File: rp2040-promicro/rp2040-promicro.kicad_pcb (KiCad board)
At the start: 2 copper layers, 17.8 x 35.6 mm, 32 parts, among them J1 USB2.0_C_v3, J2 ProMicro-LeftPin, J3 ProMicro-RightPin, SW1 SW_Push, U1 RP2040, U2 W25Q128JVS, U3 AZ1117-3.3, Y1 Crystal_GND24

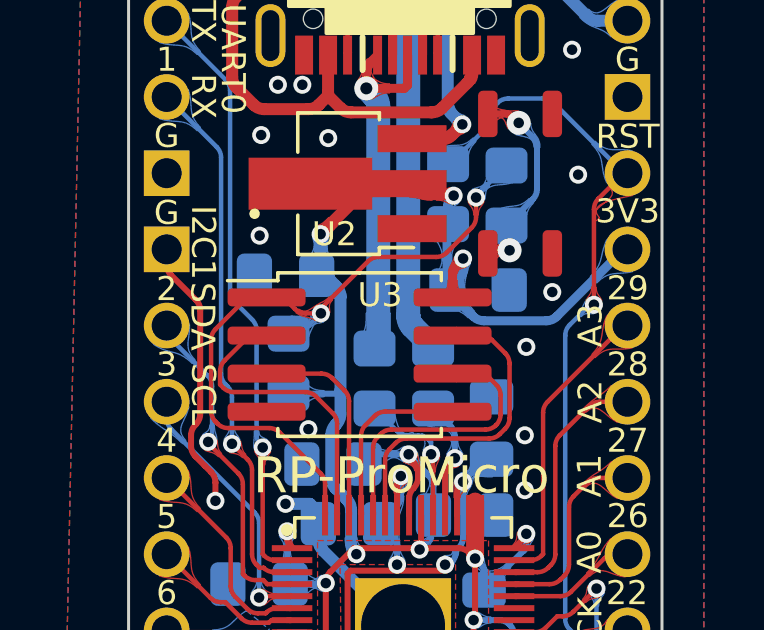
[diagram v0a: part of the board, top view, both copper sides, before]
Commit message: rp-promicro v2.0.0
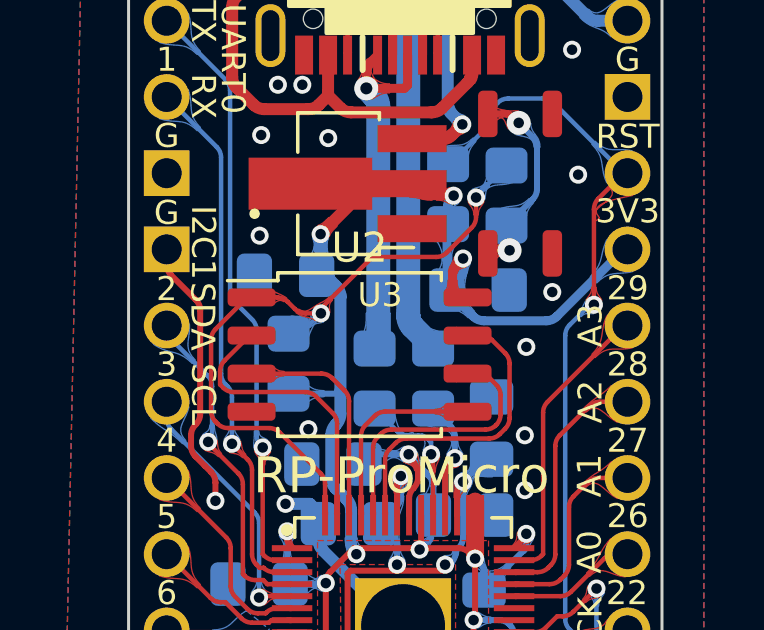
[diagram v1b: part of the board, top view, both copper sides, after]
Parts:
- U2: footprint rp2040-dev-board:W25Q16-128JV-SOIC -> Package_SO:SOIC-8_5.23x5.23mm_P1.27mm
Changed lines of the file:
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@@
     (descr "RP 2040")
     (tags "Integrated Circuit")
+    (property "MPN" "C2040")
     (property "Sheetfile" "rp2040-promicro.kicad_sch")
     (property "Sheetname" "")
@@
       (net 11 "9{slash}RX1") (pinfunction "9/A9") (pintype "bidirectional"))
   )
-  (footprint "rp2040-dev-board:W25Q16-128JV-SOIC" (layer "F.Cu")
+  (footprint "Package_SO:SOIC-8_5.23x5.23mm_P1.27mm" (layer "F.Cu")
     (at 57.7 62.397)
     (descr "SOIC, 8 Pin (http://www.winbond.com/resource-files/w25q32jv%20revg%2003272018%20plus.pdf#page=68), generated with kicad-footprint-generator ipc_gullwing_generator.py")
@@
     (property "Sheetname" "")
     (attr smd)
-    (fp_text reference "U2" (at -0.842 -4.015) (layer "F.SilkS")
-      (effects (font (size 0.8 0.8) (thickness 0.12)))
+    (fp_text reference "U2" (at 0 -3.56) (layer "F.SilkS")
+      (effects (font (size 1 1) (thickness 0.15)))
     )
     (fp_text value "W25Q128JVS" (at 0 3.56) (layer "F.Fab")
@@
       (effects (font (size 1 1) (thickness 0.15)))
     )
+    (fp_line (start -2.725 -2.725) (end -2.725 -2.465) (layer "F.SilkS") (width 0.12))
+    (fp_line (start 2.725 -2.725) (end 2.725 -2.465) (layer "F.SilkS") (width 0.12))
+    (fp_line (start 0 2.725) (end -2.725 2.725) (layer "F.SilkS") (width 0.12))
+    (fp_line (start -2.725 2.725) (end -2.725 2.465) (layer "F.SilkS") (width 0.12))
+    (fp_line (start -2.725 -2.465) (end -4.4 -2.465) (layer "F.SilkS") (width 0.12))
+    (fp_line (start 0 -2.725) (end -2.725 -2.725) (layer "F.SilkS") (width 0.12))
+    (fp_line (start 0 -2.725) (end 2.725 -2.725) (layer "F.SilkS") (width 0.12))
+    (fp_line (start 0 2.725) (end 2.725 2.725) (layer "F.SilkS") (width 0.12))
     (fp_line (start 2.725 2.725) (end 2.725 2.465) (layer "F.SilkS") (width 0.12))
-    (fp_line (start -2.725 -2.465) (end -4.4 -2.465) (layer "F.SilkS") (width 0.12))
-    (fp_line (start 0 -2.725) (end 2.725 -2.725) (layer "F.SilkS") (width 0.12))
-    (fp_line (start -2.725 2.725) (end -2.725 2.465) (layer "F.SilkS") (width 0.12))
-    (fp_line (start 2.725 -2.725) (end 2.725 -2.465) (layer "F.SilkS") (width 0.12))
-    (fp_line (start 0 -2.725) (end -2.725 -2.725) (layer "F.SilkS") (width 0.12))
-    (fp_line (start 0 2.725) (end -2.725 2.725) (layer "F.SilkS") (width 0.12))
-    (fp_line (start -2.725 -2.725) (end -2.725 -2.465) (layer "F.SilkS") (width 0.12))
-    (fp_line (start 0 2.725) (end 2.725 2.725) (layer "F.SilkS") (width 0.12))
+    (fp_line (start 4.65 2.86) (end 4.65 -2.86) (layer "F.CrtYd") (width 0.05))
+    (fp_line (start -4.65 2.86) (end 4.65 2.86) (layer "F.CrtYd") (width 0.05))
+    (fp_line (start 4.65 -2.86) (end -4.65 -2.86) (layer "F.CrtYd") (width 0.05))
     (fp_line (start -4.65 -2.86) (end -4.65 2.86) (layer "F.CrtYd") (width 0.05))
-    (fp_line (start 4.65 -2.86) (end -4.65 -2.86) (layer "F.CrtYd") (width 0.05))
-    (fp_line (start -4.65 2.86) (end 4.65 2.86) (layer "F.CrtYd") (width 0.05))
-    (fp_line (start 4.65 2.86) (end 4.65 -2.86) (layer "F.CrtYd") (width 0.05))
+    (fp_line (start -2.615 2.615) (end -2.615 -1.615) (layer "F.Fab") (width 0.1))
+    (fp_line (start 2.615 2.615) (end -2.615 2.615) (layer "F.Fab") (width 0.1))
     (fp_line (start -2.615 -1.615) (end -1.615 -2.615) (layer "F.Fab") (width 0.1))
+    (fp_line (start -1.615 -2.615) (end 2.615 -2.615) (layer "F.Fab") (width 0.1))
     (fp_line (start 2.615 -2.615) (end 2.615 2.615) (layer "F.Fab") (width 0.1))
-    (fp_line (start 2.615 2.615) (end -2.615 2.615) (layer "F.Fab") (width 0.1))
-    (fp_line (start -1.6 2.615) (end -1.6 -2.615) (layer "F.Fab") (width 0.1))
-    (fp_line (start -2.615 2.615) (end -2.615 -1.615) (layer "F.Fab") (width 0.1))
-    (fp_line (start -1.615 -2.615) (end 2.615 -2.615) (layer "F.Fab") (width 0.1))
-    (fp_line (start 1.6 2.615) (end 1.6 -2.615) (layer "F.Fab") (width 0.1))
-    (pad "1" smd roundrect (at -3.1 -1.905) (size 2.6 0.6) (layers "F.Cu" "F.Paste" "F.Mask") (roundrect_rratio 0.25)
+    (pad "1" smd roundrect locked (at -3.6 -1.905) (size 1.6 0.6) (layers "F.Cu" "F.Paste" "F.Mask") (roundrect_rratio 0.25)
       (net 1 "QSPI_SS") (pinfunction "~{CS}") (pintype "input"))
-    (pad "2" smd roundrect (at -3.1 -0.635) (size 2.6 0.6) (layers "F.Cu" "F.Paste" "F.Mask") (roundrect_rratio 0.25)
+    (pad "2" smd roundrect locked (at -3.6 -0.635) (size 1.6 0.6) (layers "F.Cu" "F.Paste" "F.Mask") (roundrect_rratio 0.25)
       (net 2 "QSPI_SD1") (pinfunction "DO(IO1)") (pintype "bidirectional"))
-    (pad "3" smd roundrect (at -3.1 0.635) (size 2.6 0.6) (layers "F.Cu" "F.Paste" "F.Mask") (roundrect_rratio 0.25)
+    (pad "3" smd roundrect locked (at -3.6 0.635) (size 1.6 0.6) (layers "F.Cu" "F.Paste" "F.Mask") (roundrect_rratio 0.25)
       (net 3 "QSPI_SD2") (pinfunction "IO2") (pintype "bidirectional"))
-    (pad "4" smd roundrect (at -3.1 1.905) (size 2.6 0.6) (layers "F.Cu" "F.Paste" "F.Mask") (roundrect_rratio 0.25)
-      (net 4 "GND") (pinfunction "GND") (pintype "power_in") (zone_connect 2))
-    (pad "5" smd roundrect (at 3.1 1.905) (size 2.6 0.6) (layers "F.Cu" "F.Paste" "F.Mask") (roundrect_rratio 0.25)
+    (pad "4" smd roundrect locked (at -3.6 1.905) (size 1.6 0.6) (layers "F.Cu" "F.Paste" "F.Mask") (roundrect_rratio 0.25)
+      (net 4 "GND") (pinfunction "GND") (pintype "power_in"))
+    (pad "5" smd roundrect locked (at 3.6 1.905) (size 1.6 0.6) (layers "F.Cu" "F.Paste" "F.Mask") (roundrect_rratio 0.25)
       (net 5 "QSPI_SD0") (pinfunction "DI(IO0)") (pintype "bidirectional"))
-    (pad "6" smd roundrect (at 3.1 0.635) (size 2.6 0.6) (layers "F.Cu" "F.Paste" "F.Mask") (roundrect_rratio 0.25)
+    (pad "6" smd roundrect locked (at 3.6 0.635) (size 1.6 0.6) (layers "F.Cu" "F.Paste" "F.Mask") (roundrect_rratio 0.25)
       (net 6 "QSPI_CLK") (pinfunction "CLK") (pintype "input"))
-    (pad "7" smd roundrect (at 3.1 -0.635) (size 2.6 0.6) (layers "F.Cu" "F.Paste" "F.Mask") (roundrect_rratio 0.25)
+    (pad "7" smd roundrect locked (at 3.6 -0.635) (size 1.6 0.6) (layers "F.Cu" "F.Paste" "F.Mask") (roundrect_rratio 0.25)
       (net 7 "QSPI_SD3") (pinfunction "IO3") (pintype "bidirectional"))
-    (pad "8" smd roundrect (at 3.1 -1.905) (size 2.6 0.6) (layers "F.Cu" "F.Paste" "F.Mask") (roundrect_rratio 0.25)
+    (pad "8" smd roundrect locked (at 3.6 -1.905) (size 1.6 0.6) (layers "F.Cu" "F.Paste" "F.Mask") (roundrect_rratio 0.25)
       (net 45 "+3V3") (pinfunction "VCC") (pintype "power_in"))
-    (model "${KICAD6_3DMODEL_DIR}/Package_SO.3dshapes/SOIC-8_5.275x5.275mm_P1.27mm.wrl"
+    (model "${KICAD6_3DMODEL_DIR}/Package_SO.3dshapes/SOIC-8_5.23x5.23mm_P1.27mm.wrl"
       (offset (xyz 0 0 0))
       (scale (xyz 1 1 1))

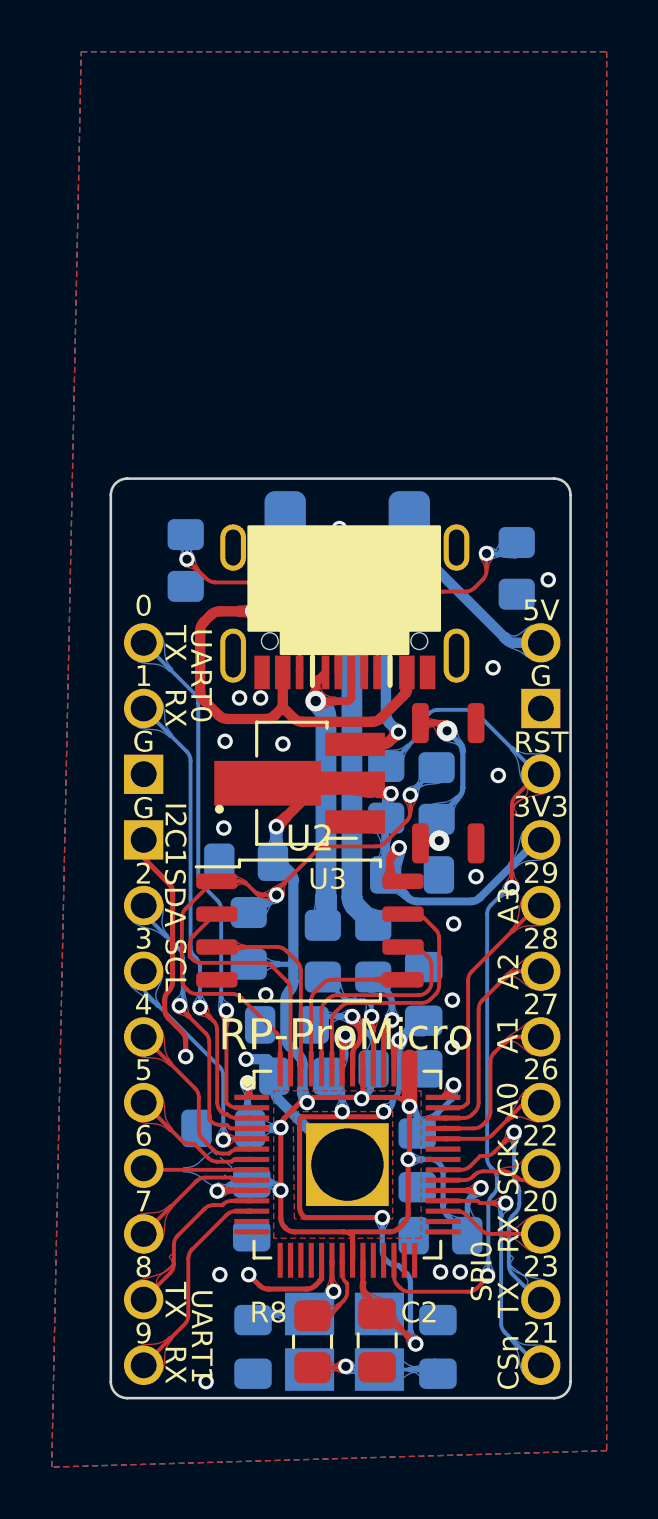
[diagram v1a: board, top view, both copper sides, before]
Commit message: rp-promicro v2.0.0
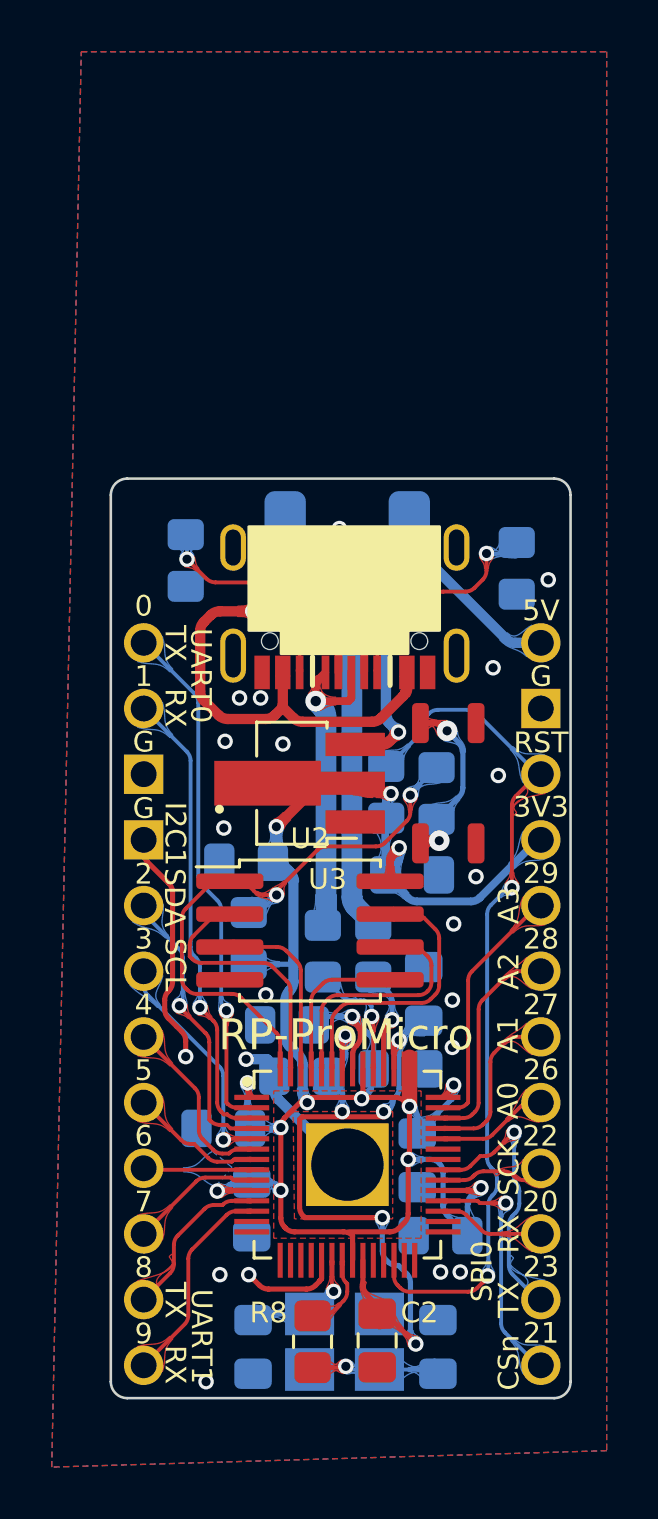
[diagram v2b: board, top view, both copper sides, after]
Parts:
- U2: footprint Package_SO:SOIC-8_5.23x5.23mm_P1.27mm -> $74th:W25Q16-128JV-SOIC

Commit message: rp2040-promicro/2.0.1
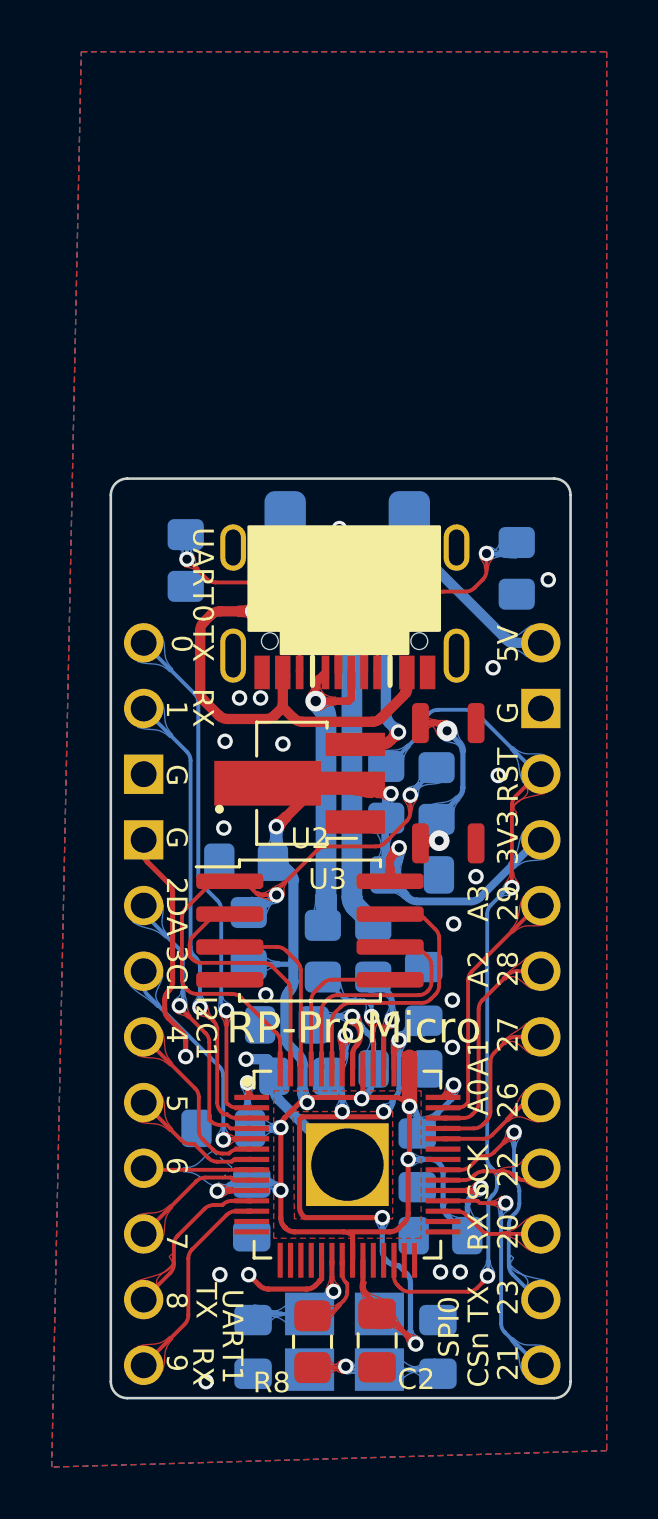
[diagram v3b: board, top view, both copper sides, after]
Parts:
- added G***: LOGO, $74th:74th-3mm, B.Cu at (64.5, 54.3)
- added REF**: twitter, $74th:twitter, F.Cu at (55.9, 56.8)
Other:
- board text added: "2DA"
- board text added: "3CL"
- board text added: "v2.0.1"
- board text removed: "2"
- board text removed: "3"
- board text removed: "SCL"
- board text removed: "SDA"
- board text removed: "v2.0.0"
